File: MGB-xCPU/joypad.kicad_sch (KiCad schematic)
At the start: 12 parts, among them SW2 LEFT, SW3 UP, SW4 DOWN, SW5 RIGHT, SW6 SELECT, SW7 START, SW8 B, SW9 A

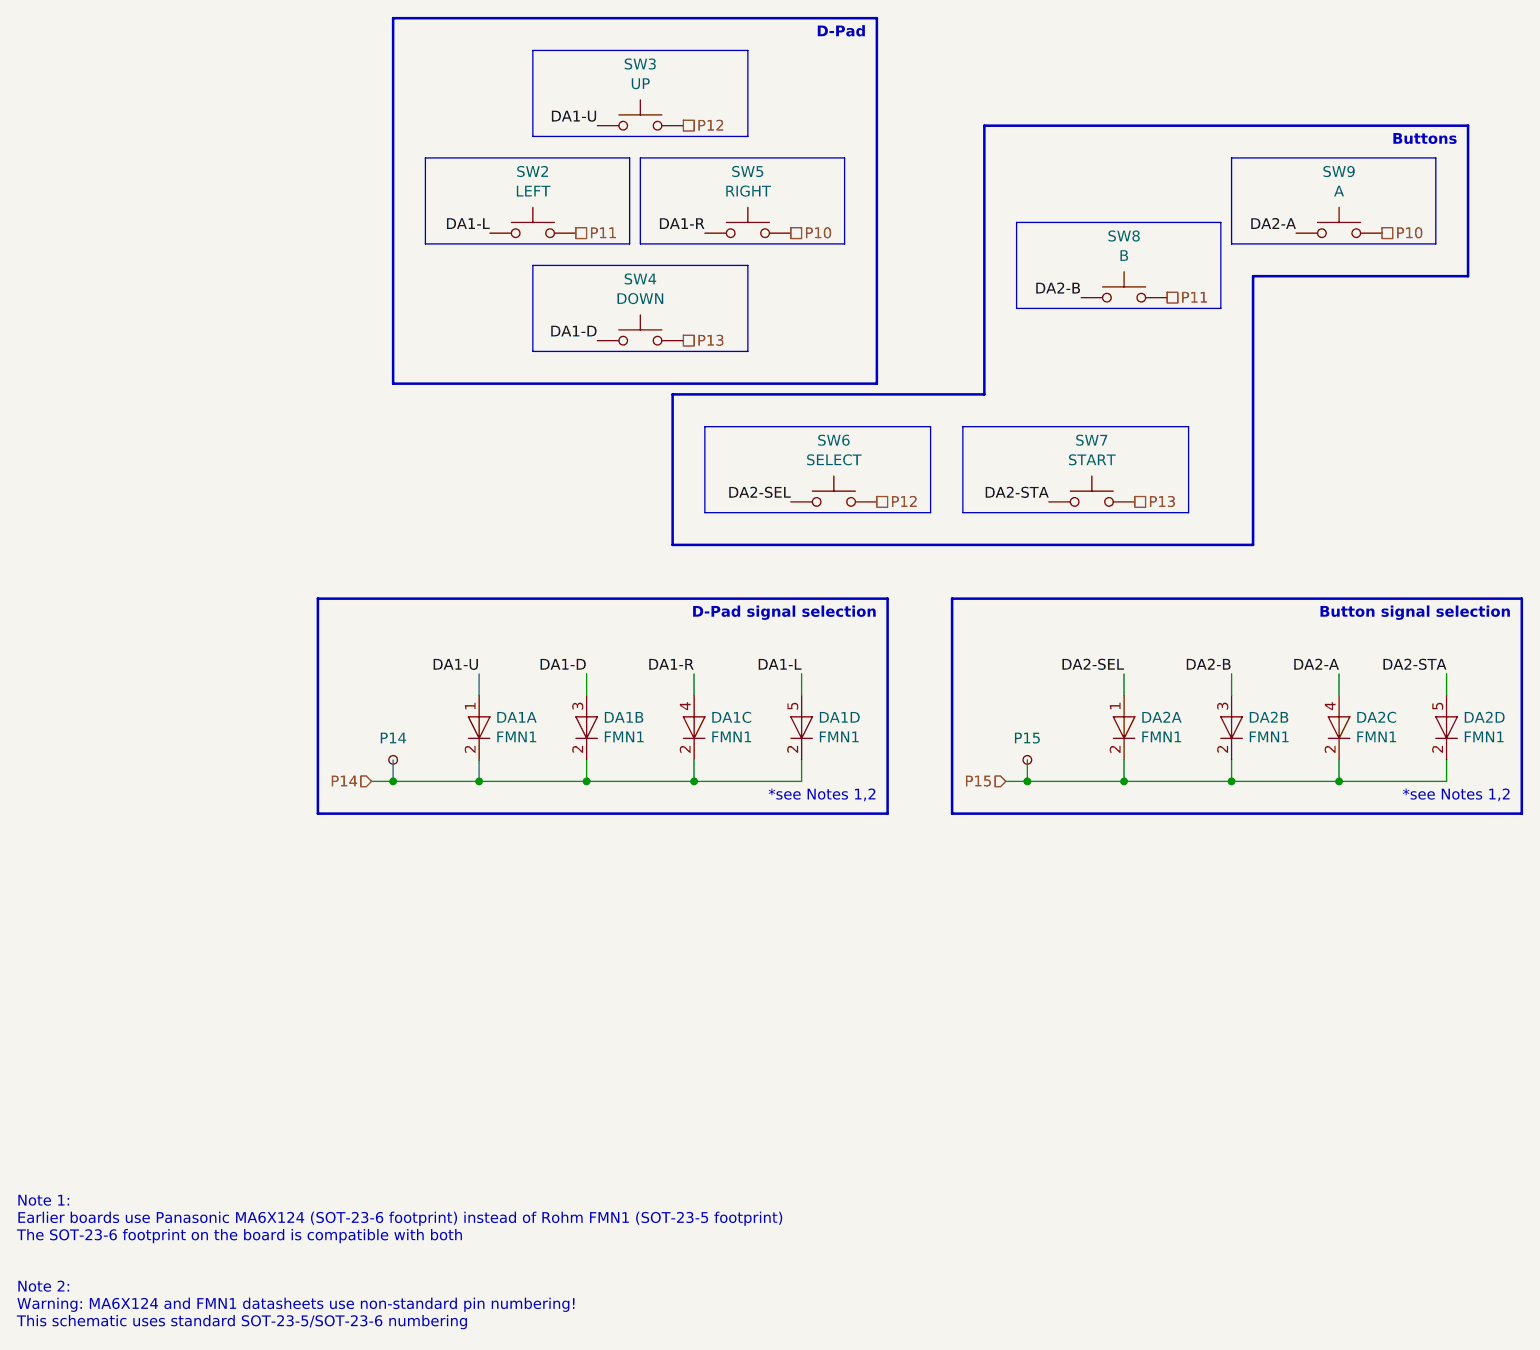
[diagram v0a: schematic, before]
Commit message: Update to latest KiCad
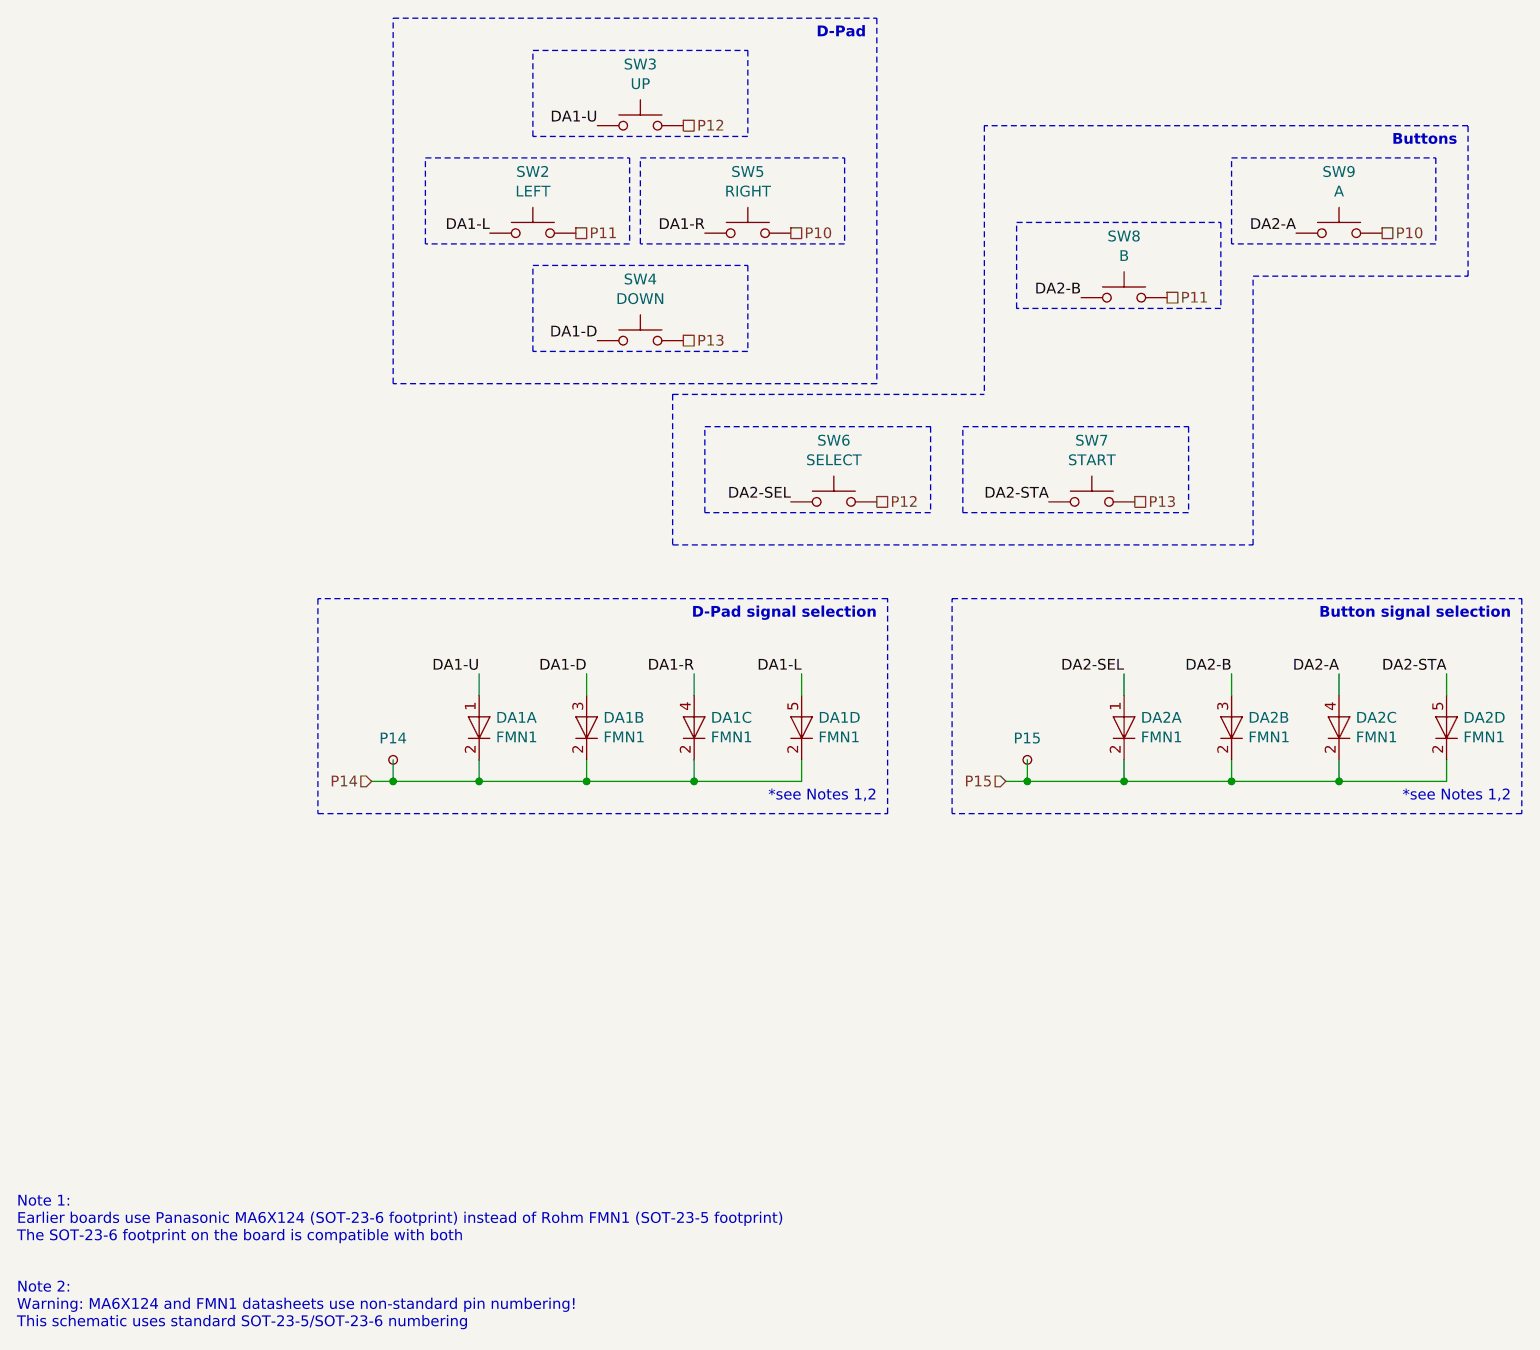
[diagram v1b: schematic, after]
